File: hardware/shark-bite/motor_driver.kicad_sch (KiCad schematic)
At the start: 42 parts, among them U10 IRFH7440TRPBF, U11 IRFH7440TRPBF, U12 IRFH7440TRPBF, U4 GD32E230G6U6TR, U5 FD6288Q, U6 AOZ1282CI, U7 IRFH7440TRPBF, U8 IRFH7440TRPBF, U9 IRFH7440TRPBF

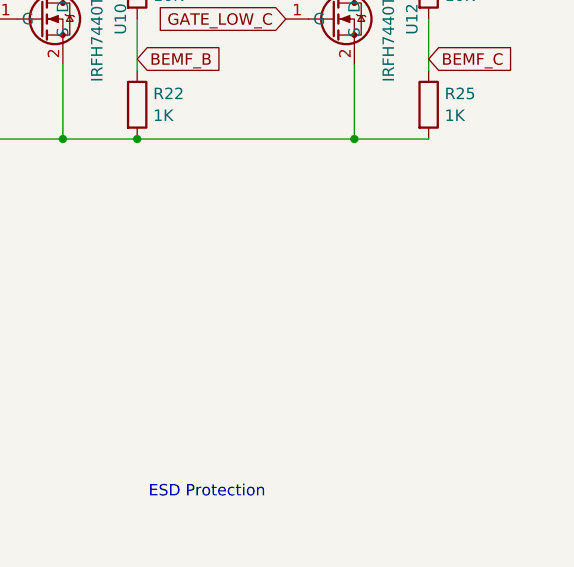
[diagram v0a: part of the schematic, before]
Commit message: Routed Without Debug
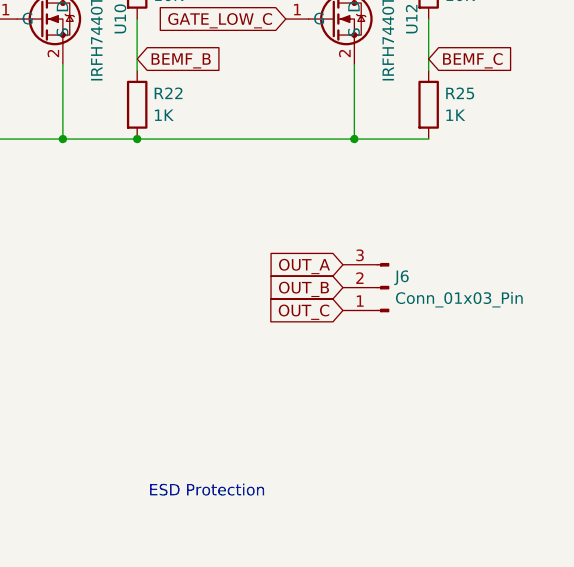
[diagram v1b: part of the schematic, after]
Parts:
- added J6: Conn_01x03_Pin, Sharkbite:ESC Pads, symbol Connector:Conn_01x03_Pin
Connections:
- net OUT_A: now also J6.3 (Pin_3)
- net OUT_B: now also J6.2 (Pin_2)
- net OUT_C: now also J6.1 (Pin_1)
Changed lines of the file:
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@@
+    )
+  )
+  (global_label "OUT_B" (shape input) (at 257.81 98.425 180) (fields_autoplaced)
+    (effects (font (size 1.27 1.27)) (justify right))
+    (property "Intersheetrefs" "${INTERSHEET_REFS}" (at 248.8635 98.425 0)
+      (effects (font (size 1.27 1.27)) (justify right) hide)
     )
   )
@@
     )
   )
+  (global_label "OUT_A" (shape input) (at 257.81 95.885 180) (fields_autoplaced)
+    (effects (font (size 1.27 1.27)) (justify right))
+    (property "Intersheetrefs" "${INTERSHEET_REFS}" (at 249.0449 95.885 0)
+      (effects (font (size 1.27 1.27)) (justify right) hide)
+    )
+  )
   (global_label "OUT_B" (shape input) (at 93.345 152.4 0) (fields_autoplaced)
     (effects (font (size 1.27 1.27)) (justify left))
@@
     (property "Intersheetrefs" "${INTERSHEET_REFS}" (at 78.1011 65.405 0)
       (effects (font (size 1.27 1.27)) (justify left) hide)
+    )
+  )
+  (global_label "OUT_C" (shape input) (at 257.81 100.965 180) (fields_autoplaced)
+    (effects (font (size 1.27 1.27)) (justify right))
+    (property "Intersheetrefs" "${INTERSHEET_REFS}" (at 248.8635 100.965 0)
+      (effects (font (size 1.27 1.27)) (justify right) hide)
     )
   )
@@
         )
       )
+    )
+  )
+  (symbol (lib_id "Connector:Conn_01x03_Pin") (at 262.89 98.425 180) (unit 1)
+    (in_bom yes) (on_board yes) (dnp no) (fields_autoplaced)
+    (property "Reference" "J6" (at 263.6012 97.2129 0)
+      (effects (font (size 1.27 1.27)) (justify right))
+    )
+    (property "Value" "Conn_01x03_Pin" (at 263.6012 99.6371 0)
+      (effects (font (size 1.27 1.27)) (justify right))
+    )
+    (property "Footprint" "Sharkbite:ESC Pads" (at 262.89 98.425 0)
+      (effects (font (size 1.27 1.27)) hide)
+    )
+    (property "Datasheet" "~" (at 262.89 98.425 0)
+      (effects (font (size 1.27 1.27)) hide)
+    )
+    (pin "1")
+    (pin "2")
+    (pin "3")
+    (instances
+      (project "malenki-hv"
+        (path "/f41619e3-8cf2-4511-8a51-762d4de43197/b339fba4-a8e4-4c66-ad9c-610bd968ae93"
+          (reference "J6") (unit 1)
+        )
+      )
